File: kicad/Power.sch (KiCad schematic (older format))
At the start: 11 parts, among them U3 LXDC2UR30

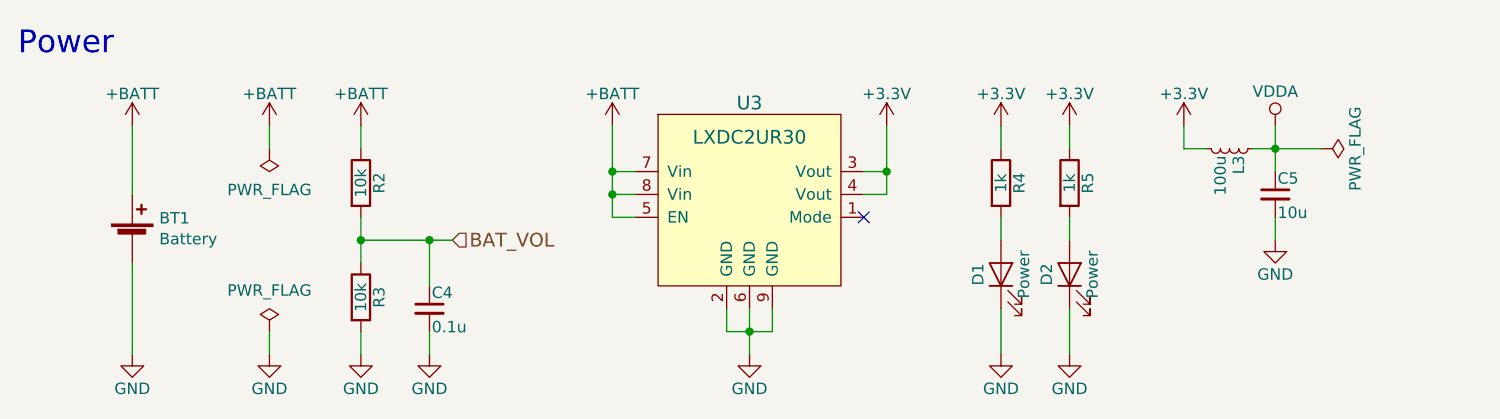
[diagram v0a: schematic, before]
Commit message: コンデンサを追加
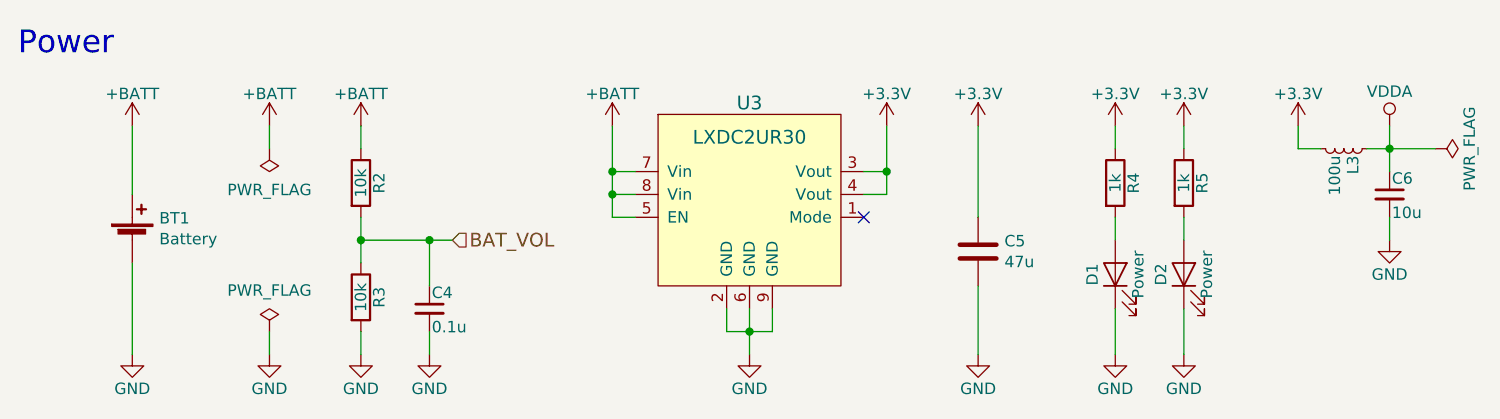
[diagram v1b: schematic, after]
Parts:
- added C5: 47u, Capacitors_SMD:C_0805, symbol Device:C
- renumbered C5 to C6
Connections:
- net +3V3: now also C5.1
- net GND: now also C5.2
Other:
- moved on the sheet: C6, D1, D2, L3, R4, R5
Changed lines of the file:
@@
 L Device:R R4
 U 1 1 57D00960
-P 5800 4450
-F 0 "R4" V 5880 4450 50  0000 C CNN
-F 1 "1k" V 5800 4450 50  0000 C CNN
-F 2 "Resistors_SMD:R_0201_NoSilk" V 5730 4450 50  0001 C CNN
-F 3 "" H 5800 4450 50  0000 C CNN
-	1    5800 4450
-	1    0    0    -1
-$EndComp
-$Comp
-L power:GND #PWR027
+P 6300 4450
+F 0 "R4" V 6380 4450 50  0000 C CNN
+F 1 "1k" V 6300 4450 50  0000 C CNN
+F 2 "Resistors_SMD:R_0201_NoSilk" V 6230 4450 50  0001 C CNN
+F 3 "" H 6300 4450 50  0000 C CNN
+	1    6300 4450
+	1    0    0    -1
+$EndComp
+$Comp
+L power:GND #PWR029
 U 1 1 57D00A42
-P 5800 5200
-F 0 "#PWR027" H 5800 4950 50  0001 C CNN
-F 1 "GND" H 5800 5050 50  0000 C CNN
-F 2 "" H 5800 5200 50  0000 C CNN
-F 3 "" H 5800 5200 50  0000 C CNN
-	1    5800 5200
+P 6300 5200
+F 0 "#PWR029" H 6300 4950 50  0001 C CNN
+F 1 "GND" H 6300 5050 50  0000 C CNN
+F 2 "" H 6300 5200 50  0000 C CNN
+F 3 "" H 6300 5200 50  0000 C CNN
+	1    6300 5200
 	1    0    0    -1
 $EndComp
@@
 $EndComp
 $Comp
-L power:+3.3V #PWR026
+L power:+3.3V #PWR028
 U 1 1 589CB64F
-P 5800 4200
-F 0 "#PWR026" H 5800 4050 50  0001 C CNN
-F 1 "+3.3V" H 5800 4340 50  0000 C CNN
-F 2 "" H 5800 4200 50  0000 C CNN
-F 3 "" H 5800 4200 50  0000 C CNN
-	1    5800 4200
+P 6300 4200
+F 0 "#PWR028" H 6300 4050 50  0001 C CNN
+F 1 "+3.3V" H 6300 4340 50  0000 C CNN
+F 2 "" H 6300 4200 50  0000 C CNN
+F 3 "" H 6300 4200 50  0000 C CNN
+	1    6300 4200
 	1    0    0    -1
 $EndComp
@@
 	2600 4200 2600 4300
 Wire Wire Line
-	5800 4700 5800 4600
-Wire Wire Line
-	5800 4300 5800 4200
+	6300 4700 6300 4600
+Wire Wire Line
+	6300 4300 6300 4200
 Wire Wire Line
 	4200 4500 4100 4500
@@
 L Device:LED D1
 U 1 1 594AB638
-P 5800 4850
-F 0 "D1" H 5800 4950 50  0000 C CNN
-F 1 "Power" H 5800 4750 50  0000 C CNN
-F 2 "LEDs:LED_0402" H 5800 4850 50  0001 C CNN
-F 3 "" H 5800 4850 50  0001 C CNN
-	1    5800 4850
+P 6300 4850
+F 0 "D1" H 6300 4950 50  0000 C CNN
+F 1 "Power" H 6300 4750 50  0000 C CNN
+F 2 "LEDs:LED_0402" H 6300 4850 50  0001 C CNN
+F 3 "" H 6300 4850 50  0001 C CNN
+	1    6300 4850
 	0    -1   -1   0
 $EndComp
 Wire Wire Line
-	5800 5000 5800 5200
-$Comp
-L power:+3.3V #PWR030
+	6300 5000 6300 5200
+$Comp
+L power:+3.3V #PWR032
 U 1 1 59C37023
-P 6600 4200
-F 0 "#PWR030" H 6600 4050 50  0001 C CNN
-F 1 "+3.3V" H 6600 4340 50  0000 C CNN
-F 2 "" H 6600 4200 50  0001 C CNN
-F 3 "" H 6600 4200 50  0001 C CNN
-	1    6600 4200
+P 7100 4200
+F 0 "#PWR032" H 7100 4050 50  0001 C CNN
+F 1 "+3.3V" H 7100 4340 50  0000 C CNN
+F 2 "" H 7100 4200 50  0001 C CNN
+F 3 "" H 7100 4200 50  0001 C CNN
+	1    7100 4200
 	1    0    0    -1
 $EndComp
@@
 L Device:L_Small L3
 U 1 1 59C3706B
-P 6800 4300
-F 0 "L3" H 6830 4340 50  0000 L CNN
-F 1 "100u" H 6830 4260 50  0000 L CNN
-F 2 "Capacitors_SMD:C_0603" H 6800 4300 50  0001 C CNN
-F 3 "" H 6800 4300 50  0001 C CNN
-	1    6800 4300
+P 7300 4300
+F 0 "L3" H 7330 4340 50  0000 L CNN
+F 1 "100u" H 7330 4260 50  0000 L CNN
+F 2 "Capacitors_SMD:C_0603" H 7300 4300 50  0001 C CNN
+F 3 "" H 7300 4300 50  0001 C CNN
+	1    7300 4300
 	0    1    1    0
 $EndComp
 $Comp
-L Device:C_Small C5
+L Device:C_Small C6
 U 1 1 59C370C1
-P 7000 4500
-F 0 "C5" H 7010 4570 50  0000 L CNN
-F 1 "10u" H 7010 4420 50  0000 L CNN
-F 2 "Capacitors_SMD:C_0402_NoSilk" H 7000 4500 50  0001 C CNN
-F 3 "" H 7000 4500 50  0001 C CNN
-	1    7000 4500
-	1    0    0    -1
-$EndComp
-Wire Wire Line
-	7000 4200 7000 4300
-$Comp
-L power:GND #PWR032
+P 7500 4500
+F 0 "C6" H 7510 4570 50  0000 L CNN
+F 1 "10u" H 7510 4420 50  0000 L CNN
+F 2 "Capacitors_SMD:C_0402_NoSilk" H 7500 4500 50  0001 C CNN
+F 3 "" H 7500 4500 50  0001 C CNN
+	1    7500 4500
+	1    0    0    -1
+$EndComp
+Wire Wire Line
+	7500 4200 7500 4300
+$Comp
+L power:GND #PWR034
 U 1 1 59C37170
-P 7000 4700
-F 0 "#PWR032" H 7000 4450 50  0001 C CNN
-F 1 "GND" H 7000 4550 50  0000 C CNN
-F 2 "" H 7000 4700 50  0000 C CNN
-F 3 "" H 7000 4700 50  0000 C CNN
-	1    7000 4700
-	1    0    0    -1
-$EndComp
-Wire Wire Line
-	7000 4700 7000 4600
-Wire Wire Line
-	6900 4300 7000 4300
-Connection ~ 7000 4300
-Wire Wire Line
-	6700 4300 6600 4300
-Wire Wire Line
-	6600 4300 6600 4200
+P 7500 4700
+F 0 "#PWR034" H 7500 4450 50  0001 C CNN
+F 1 "GND" H 7500 4550 50  0000 C CNN
+F 2 "" H 7500 4700 50  0000 C CNN
+F 3 "" H 7500 4700 50  0000 C CNN
+	1    7500 4700
+	1    0    0    -1
+$EndComp
+Wire Wire Line
+	7500 4700 7500 4600
+Wire Wire Line
+	7400 4300 7500 4300
+Connection ~ 7500 4300
+Wire Wire Line
+	7200 4300 7100 4300
+Wire Wire Line
+	7100 4300 7100 4200
 $Comp
 L Device:C_Small C4
@@
 L power:PWR_FLAG #FLG03
 U 1 1 5A1BE075
-P 7200 4300
-F 0 "#FLG03" H 7200 4375 50  0001 C CNN
-F 1 "PWR_FLAG" H 7200 4450 50  0000 C CNN
-F 2 "" H 7200 4300 50  0001 C CNN
-F 3 "" H 7200 4300 50  0001 C CNN
-	1    7200 4300
+P 7700 4300
+F 0 "#FLG03" H 7700 4375 50  0001 C CNN
+F 1 "PWR_FLAG" H 7700 4450 50  0000 C CNN
+F 2 "" H 7700 4300 50  0001 C CNN
+F 3 "" H 7700 4300 50  0001 C CNN
+	1    7700 4300
 	0    1    1    0
 $EndComp
@@
 L Device:R R5
 U 1 1 5A4BB521
-P 6100 4450
-F 0 "R5" V 6180 4450 50  0000 C CNN
-F 1 "1k" V 6100 4450 50  0000 C CNN
-F 2 "Resistors_SMD:R_0201_NoSilk" V 6030 4450 50  0001 C CNN
-F 3 "" H 6100 4450 50  0000 C CNN
-	1    6100 4450
-	1    0    0    -1
-$EndComp
-$Comp
-L power:GND #PWR029
+P 6600 4450
+F 0 "R5" V 6680 4450 50  0000 C CNN
+F 1 "1k" V 6600 4450 50  0000 C CNN
+F 2 "Resistors_SMD:R_0201_NoSilk" V 6530 4450 50  0001 C CNN
+F 3 "" H 6600 4450 50  0000 C CNN
+	1    6600 4450
+	1    0    0    -1
+$EndComp
+$Comp
+L power:GND #PWR031
 U 1 1 5A4BB527
-P 6100 5200
-F 0 "#PWR029" H 6100 4950 50  0001 C CNN
-F 1 "GND" H 6100 5050 50  0000 C CNN
-F 2 "" H 6100 5200 50  0000 C CNN
-F 3 "" H 6100 5200 50  0000 C CNN
-	1    6100 5200
-	1    0    0    -1
-$EndComp
-$Comp
-L power:+3.3V #PWR028
+P 6600 5200
+F 0 "#PWR031" H 6600 4950 50  0001 C CNN
+F 1 "GND" H 6600 5050 50  0000 C CNN
+F 2 "" H 6600 5200 50  0000 C CNN
+F 3 "" H 6600 5200 50  0000 C CNN
+	1    6600 5200
+	1    0    0    -1
+$EndComp
+$Comp
+L power:+3.3V #PWR030
 U 1 1 5A4BB52D
-P 6100 4200
-F 0 "#PWR028" H 6100 4050 50  0001 C CNN
-F 1 "+3.3V" H 6100 4340 50  0000 C CNN
-F 2 "" H 6100 4200 50  0000 C CNN
-F 3 "" H 6100 4200 50  0000 C CNN
-	1    6100 4200
-	1    0    0    -1
-$EndComp
-Wire Wire Line
-	6100 4700 6100 4600
-Wire Wire Line
-	6100 4300 6100 4200
+P 6600 4200
+F 0 "#PWR030" H 6600 4050 50  0001 C CNN
+F 1 "+3.3V" H 6600 4340 50  0000 C CNN
+F 2 "" H 6600 4200 50  0000 C CNN
+F 3 "" H 6600 4200 50  0000 C CNN
+	1    6600 4200
+	1    0    0    -1
+$EndComp
+Wire Wire Line
+	6600 4700 6600 4600
+Wire Wire Line
+	6600 4300 6600 4200
 $Comp
 L Device:LED D2
 U 1 1 5A4BB535
-P 6100 4850
-F 0 "D2" H 6100 4950 50  0000 C CNN
-F 1 "Power" H 6100 4750 50  0000 C CNN
-F 2 "LEDs:LED_0402" H 6100 4850 50  0001 C CNN
-F 3 "" H 6100 4850 50  0001 C CNN
-	1    6100 4850
+P 6600 4850
+F 0 "D2" H 6600 4950 50  0000 C CNN
+F 1 "Power" H 6600 4750 50  0000 C CNN
+F 2 "LEDs:LED_0402" H 6600 4850 50  0001 C CNN
+F 3 "" H 6600 4850 50  0001 C CNN
+	1    6600 4850
 	0    -1   -1   0
 $EndComp
 Wire Wire Line
-	6100 5000 6100 5200
+	6600 5000 6600 5200
 Wire Wire Line
 	5300 4400 5200 4400
@@
 	5300 4400 5300 4500
 Wire Wire Line
-	7000 4300 7000 4400
-Wire Wire Line
-	7000 4300 7200 4300
+	7500 4300 7500 4400
+Wire Wire Line
+	7500 4300 7700 4300
 Wire Wire Line
 	3300 4700 3400 4700
@@
 	2000 4500 2000 4200
 $Comp
-L power:VDDA #PWR031
+L power:VDDA #PWR033
 U 1 1 59C37047
-P 7000 4200
-F 0 "#PWR031" H 7000 4050 50  0001 C CNN
-F 1 "VDDA" H 7000 4350 50  0000 C CNN
-F 2 "" H 7000 4200 50  0001 C CNN
-F 3 "" H 7000 4200 50  0001 C CNN
-	1    7000 4200
+P 7500 4200
+F 0 "#PWR033" H 7500 4050 50  0001 C CNN
+F 1 "VDDA" H 7500 4350 50  0000 C CNN
+F 2 "" H 7500 4200 50  0001 C CNN
+F 3 "" H 7500 4200 50  0001 C CNN
+	1    7500 4200
 	1    0    0    -1
 $EndComp
@@
 	1    0    0    -1
 $EndComp
+$Comp
+L Device:C C5
+U 1 1 5B93EBC5
+P 5700 4750
+F 0 "C5" H 5815 4796 50  0000 L CNN
+F 1 "47u" H 5815 4705 50  0000 L CNN
+F 2 "Capacitors_SMD:C_0805" H 5738 4600 50  0001 C CNN
+F 3 "~" H 5700 4750 50  0001 C CNN
+	1    5700 4750
+	1    0    0    -1
+$EndComp
+$Comp
+L power:GND #PWR027
+U 1 1 5B93EC2F
+P 5700 5200
+F 0 "#PWR027" H 5700 4950 50  0001 C CNN
+F 1 "GND" H 5700 5050 50  0000 C CNN
+F 2 "" H 5700 5200 50  0000 C CNN
+F 3 "" H 5700 5200 50  0000 C CNN
+	1    5700 5200
+	1    0    0    -1
+$EndComp
+Wire Wire Line
+	5700 4900 5700 5200
+$Comp
+L power:+3.3V #PWR026
+U 1 1 5B93F57B
+P 5700 4200
+F 0 "#PWR026" H 5700 4050 50  0001 C CNN
+F 1 "+3.3V" H 5700 4340 50  0000 C CNN
+F 2 "" H 5700 4200 50  0000 C CNN
+F 3 "" H 5700 4200 50  0000 C CNN
+	1    5700 4200
+	1    0    0    -1
+$EndComp
+Wire Wire Line
+	5700 4200 5700 4600
 $EndSCHEMATC
